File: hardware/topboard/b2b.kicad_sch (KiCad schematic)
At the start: 50 parts

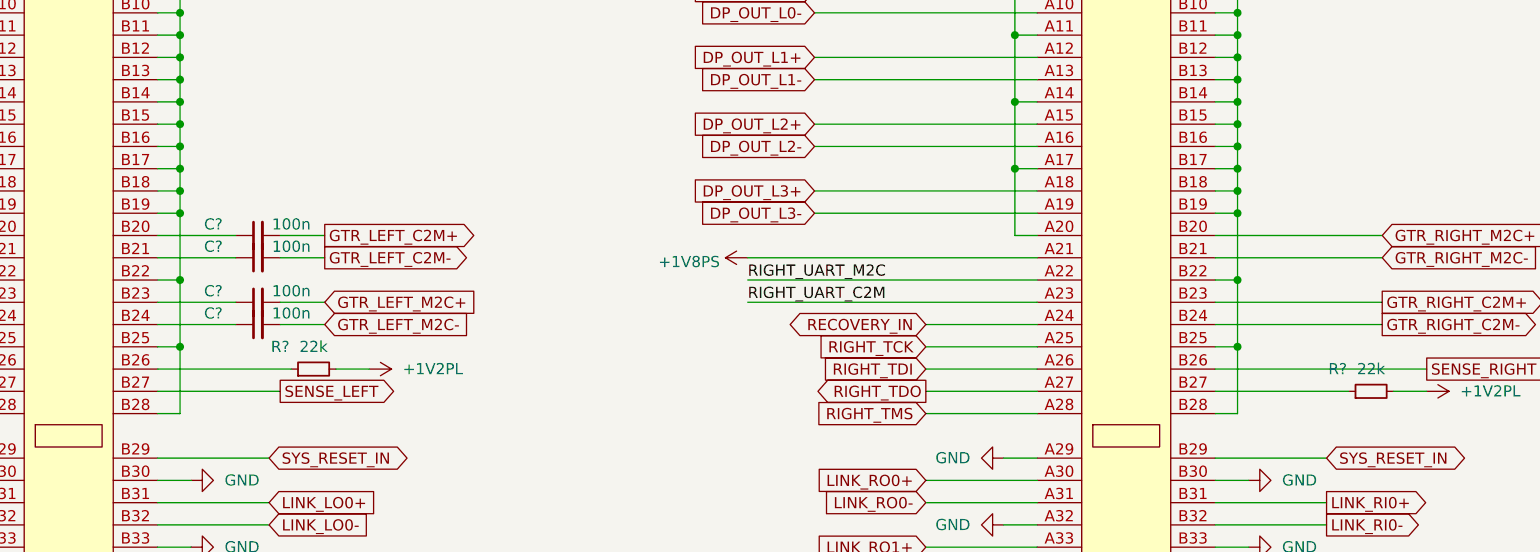
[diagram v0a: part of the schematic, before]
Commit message: Add IMU
Signed-off-by: gatecat <gatecat@ds0.me>
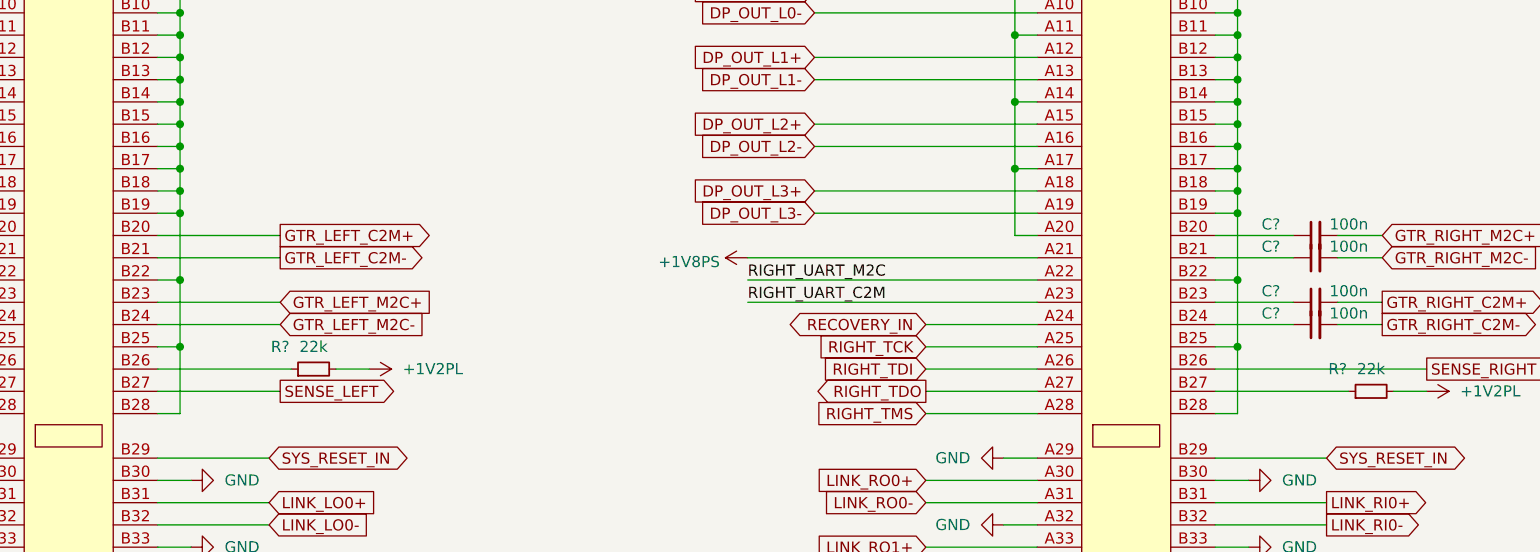
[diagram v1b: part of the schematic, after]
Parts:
- removed C? (x4): 100n, symbol Device:C_Small
- added C? (x4): 100n, symbol Device:C_Small
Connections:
- net GTR_LEFT_C2M+: now also JL.B20
- net GTR_LEFT_C2M-: now also JL.B21
- net GTR_LEFT_M2C+: now also JL.B23
- net GTR_LEFT_M2C-: now also JL.B24
- net GTR_RIGHT_C2M+: now also C?.2; no longer JL?.B23
- net GTR_RIGHT_C2M-: now also C?.2; no longer JL?.B24
- net GTR_RIGHT_M2C+: now also C?.2; no longer JL?.B20
- net GTR_RIGHT_M2C-: now also C?.2; no longer JL?.B21
- new net: C?.1, JL?.B20
- new net: C?.1, JL?.B21
- new net: C?.1, JL?.B23
- new net: C?.1, JL?.B24
